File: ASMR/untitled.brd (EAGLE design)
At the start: 91 x 91 mm, 60 parts, among them J1 U.FL-R-SMT(01), J3 2172034-1, J4 POWER_JACKSLT, Q1 MMBT3904, Q2 MMBT3904, Q3 12MHz, Q4 MC-306, U2 DS1307Z+, U3 MAX3444EASA, U4 AMS1117, U5 MAX232CSE, X1 MSTBA2

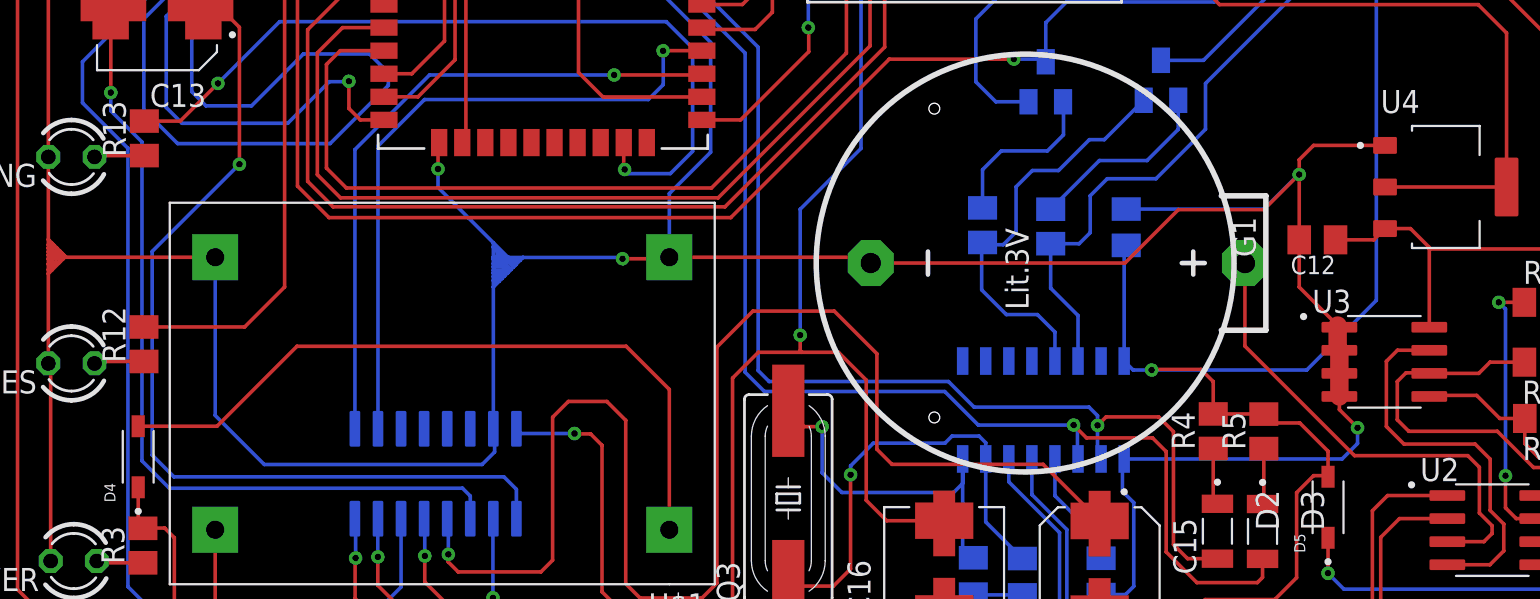
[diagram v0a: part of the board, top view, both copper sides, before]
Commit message: revisi .brd
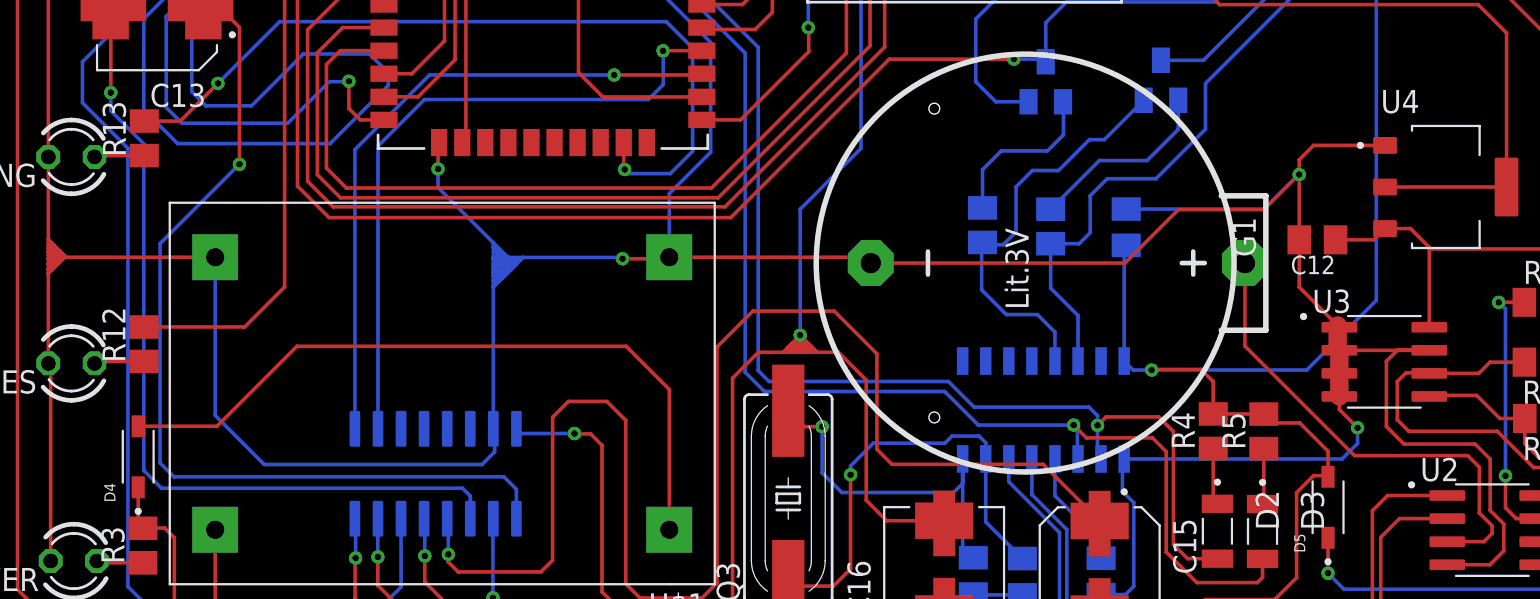
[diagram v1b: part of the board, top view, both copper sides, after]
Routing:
- net 3V3: track 234.7 -> 243.0 mm
- net GND: track 632.6 -> 636.9 mm
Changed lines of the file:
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@@
 <wire x1="66.064953125" y1="16.364715625" x2="66.064953125" y2="19.9532875" width="0.2" layer="1"/>
 <wire x1="66.064953125" y1="19.9532875" x2="66.675725" y2="20.564059375" width="0.2" layer="1"/>
-<wire x1="66.675725" y1="20.564059375" x2="68.422096875" y2="20.564059375" width="0.2" layer="1"/>
+<wire x1="66.675725" y1="20.564059375" x2="67.742509375" y2="20.564059375" width="0.2" layer="1"/>
+<wire x1="67.742509375" y1="20.564059375" x2="68.422096875" y2="20.564059375" width="0.2" layer="1"/>
 <wire x1="68.422096875" y1="20.564059375" x2="68.427296875" y2="20.558859375" width="0.2" layer="1"/>
 <wire x1="46.02720625" y1="7.0947875" x2="46.02720625" y2="6.58320625" width="0.2" layer="16"/>
@@
 <wire x1="19.6946625" y1="46.11838125" x2="19.945209375" y2="46.11838125" width="0.2" layer="16"/>
 <wire x1="19.945209375" y1="46.11838125" x2="20.063746875" y2="46.23691875" width="0.2" layer="16"/>
-<wire x1="63.477296875" y1="20.558859375" x2="68.427296875" y2="20.558859375" width="0" layer="19" extent="1-1"/>
+<wire x1="63.477296875" y1="20.558859375" x2="67.737309375" y2="20.558859375" width="0.2" layer="1"/>
+<wire x1="67.737309375" y1="20.558859375" x2="67.742509375" y2="20.564059375" width="0.2" layer="1"/>
 </signal>
 <signal name="USB_P">
@@
 <wire x1="38.556709375" y1="11.177509375" x2="37.4314125" y2="12.30280625" width="0.2" layer="1"/>
 <wire x1="37.4314125" y1="18.922815625" x2="35.904071875" y2="20.45015625" width="0.2" layer="1"/>
-<wire x1="35.904071875" y1="20.45015625" x2="33.8959" y2="20.45015625" width="0.2" layer="1"/>
-<wire x1="33.8959" y1="20.45015625" x2="31.49139375" y2="20.45015625" width="0.2" layer="1"/>
+<wire x1="35.904071875" y1="20.45015625" x2="34.738465625" y2="20.45015625" width="0.2" layer="1"/>
+<wire x1="34.738465625" y1="20.45015625" x2="33.8959" y2="20.45015625" width="0.2" layer="1"/>
+<wire x1="33.8959" y1="20.45015625" x2="33.685965625" y2="20.45015625" width="0.2" layer="1"/>
+<wire x1="33.685965625" y1="20.45015625" x2="33.501034375" y2="20.45015625" width="0.2" layer="1"/>
+<wire x1="33.501034375" y1="20.45015625" x2="33.320215625" y2="20.45015625" width="0.2" layer="1"/>
+<wire x1="33.320215625" y1="20.45015625" x2="33.1846" y2="20.45015625" width="0.2" layer="1"/>
+<wire x1="33.1846" y1="20.45015625" x2="32.853134375" y2="20.45015625" width="0.2" layer="1"/>
+<wire x1="32.853134375" y1="20.45015625" x2="31.49139375" y2="20.45015625" width="0.2" layer="1"/>
 <wire x1="31.49139375" y1="20.45015625" x2="30.0717" y2="19.0304625" width="0.2" layer="1"/>
 <wire x1="30.0717" y1="19.0304625" x2="30.0717" y2="6.275275" width="0.2" layer="1"/>
@@
 <wire x1="18.4332" y1="15.97845625" x2="18.173340625" y2="16.238315625" width="0.2" layer="16"/>
 <wire x1="33.8959" y1="20.45015625" x2="33.7958" y2="20.55025625" width="0.2" layer="1"/>
-<wire x1="33.7958" y1="20.55025625" x2="33.7958" y2="21.392821875" width="0.2" layer="1"/>
+<wire x1="33.7958" y1="20.55025625" x2="33.7958" y2="20.76345625" width="0.2" layer="1"/>
 <via x="33.7958" y="21.392821875" extent="1-16" drill="0.35"/>
+<wire x1="33.7958" y1="20.76345625" x2="33.7958" y2="21.392821875" width="0.2" layer="1"/>
 <wire x1="33.7958" y1="21.392821875" x2="33.7958" y2="28.324503125" width="0.2" layer="16"/>
 <wire x1="33.7958" y1="28.324503125" x2="37.144934375" y2="31.6736375" width="0.2" layer="16"/>
@@
 <wire x1="58.911721875" y1="55.437096875" x2="58.857303125" y2="55.382678125" width="0.2" layer="1"/>
 <wire x1="58.857303125" y1="55.382678125" x2="58.857303125" y2="54.914934375" width="0.2" layer="1"/>
+<wire x1="33.7958" y1="21.392821875" x2="33.35955625" y2="20.956578125" width="0.2" layer="1"/>
+<wire x1="33.35955625" y1="20.956578125" x2="33.2712" y2="20.868221875" width="0.2" layer="1"/>
+<wire x1="33.2712" y1="20.868221875" x2="33.137640625" y2="20.7346625" width="0.2" layer="1"/>
+<wire x1="33.137640625" y1="20.7346625" x2="33.07805" y2="20.675071875" width="0.2" layer="1"/>
+<wire x1="33.07805" y1="20.675071875" x2="32.853134375" y2="20.45015625" width="0.2" layer="1"/>
+<wire x1="33.07805" y1="20.675071875" x2="33.07805" y2="20.55670625" width="0.2" layer="1"/>
+<wire x1="33.07805" y1="20.55670625" x2="33.1846" y2="20.45015625" width="0.2" layer="1"/>
+<wire x1="33.137640625" y1="20.7346625" x2="33.320215625" y2="20.5520875" width="0.2" layer="1"/>
+<wire x1="33.320215625" y1="20.5520875" x2="33.320215625" y2="20.45015625" width="0.2" layer="1"/>
+<wire x1="33.2712" y1="20.868221875" x2="33.501034375" y2="20.6383875" width="0.2" layer="1"/>
+<wire x1="33.501034375" y1="20.6383875" x2="33.501034375" y2="20.45015625" width="0.2" layer="1"/>
+<wire x1="33.35955625" y1="20.956578125" x2="33.484596875" y2="20.8315375" width="0.2" layer="1"/>
+<wire x1="33.484596875" y1="20.8315375" x2="33.56884375" y2="20.747290625" width="0.2" layer="1"/>
+<wire x1="33.56884375" y1="20.747290625" x2="33.685965625" y2="20.63016875" width="0.2" layer="1"/>
+<wire x1="33.685965625" y1="20.63016875" x2="33.685965625" y2="20.592225" width="0.2" layer="1"/>
+<wire x1="33.685965625" y1="20.592225" x2="33.685965625" y2="20.45015625" width="0.2" layer="1"/>
+<wire x1="33.7958" y1="21.392821875" x2="33.7958" y2="20.974246875" width="0.2" layer="1"/>
+<wire x1="33.56884375" y1="20.747290625" x2="33.7958" y2="20.974246875" width="0.2" layer="1"/>
+<wire x1="33.7958" y1="21.392821875" x2="33.7958" y2="21.142740625" width="0.2" layer="1"/>
+<wire x1="33.7958" y1="21.142740625" x2="33.484596875" y2="20.8315375" width="0.2" layer="1"/>
+<wire x1="33.7958" y1="21.392821875" x2="34.412409375" y2="20.7762125" width="0.2" layer="1"/>
+<wire x1="34.412409375" y1="20.7762125" x2="34.551103125" y2="20.63751875" width="0.2" layer="1"/>
+<wire x1="34.551103125" y1="20.63751875" x2="34.738465625" y2="20.45015625" width="0.2" layer="1"/>
+<wire x1="33.685965625" y1="20.592225" x2="34.505809375" y2="20.592225" width="0.2" layer="1"/>
+<wire x1="34.505809375" y1="20.592225" x2="34.551103125" y2="20.63751875" width="0.2" layer="1"/>
+<wire x1="33.7958" y1="20.76345625" x2="34.14623125" y2="20.76345625" width="0.2" layer="1"/>
+<wire x1="34.14623125" y1="20.76345625" x2="34.399653125" y2="20.76345625" width="0.2" layer="1"/>
+<wire x1="34.399653125" y1="20.76345625" x2="34.412409375" y2="20.7762125" width="0.2" layer="1"/>
+<wire x1="33.7958" y1="20.974246875" x2="33.935440625" y2="20.974246875" width="0.2" layer="1"/>
+<wire x1="33.935440625" y1="20.974246875" x2="34.14623125" y2="20.76345625" width="0.2" layer="1"/>
+<wire x1="33.7958" y1="21.392821875" x2="33.935440625" y2="21.25318125" width="0.2" layer="1"/>
+<wire x1="33.935440625" y1="21.25318125" x2="33.935440625" y2="20.974246875" width="0.2" layer="1"/>
 </signal>
 <signal name="N$12">
@@
 <wire x1="18.173340625" y1="12.908290625" x2="17.487634375" y2="13.593996875" width="0.2" layer="16"/>
 <wire x1="17.487634375" y1="13.593996875" x2="-0.6770875" y2="13.593996875" width="0.2" layer="16"/>
-<wire x1="-0.6770875" y1="13.593996875" x2="-1.87726875" y2="14.794178125" width="0.2" layer="16"/>
-<wire x1="-1.87726875" y1="14.794178125" x2="-1.87726875" y2="25.999846875" width="0.2" layer="16"/>
-<wire x1="-1.87726875" y1="25.999846875" x2="2.925103125" y2="30.80221875" width="0.2" layer="16"/>
+<wire x1="-0.6770875" y1="13.593996875" x2="-1.444428125" y2="14.3613375" width="0.2" layer="16"/>
+<wire x1="-1.444428125" y1="14.3613375" x2="-1.444428125" y2="26.4326875" width="0.2" layer="16"/>
+<wire x1="-1.444428125" y1="26.4326875" x2="2.925103125" y2="30.80221875" width="0.2" layer="16"/>
 <via x="2.925103125" y="30.80221875" extent="1-16" drill="0.35"/>
 <wire x1="2.925103125" y1="38.34308125" x2="1.9885875" y2="39.279596875" width="0.2" layer="1"/>
@@
 <wire x1="15.633340625" y1="11.288315625" x2="15.633340625" y2="12.54055625" width="0.2" layer="16"/>
 <wire x1="15.633340625" y1="12.54055625" x2="15.2060875" y2="12.967809375" width="0.2" layer="16"/>
-<wire x1="15.2060875" y1="12.967809375" x2="-0.93304375" y2="12.967809375" width="0.2" layer="16"/>
-<wire x1="-0.93304375" y1="12.967809375" x2="-2.439434375" y2="14.4742" width="0.2" layer="16"/>
-<wire x1="-2.439434375" y1="14.4742" x2="-2.439434375" y2="32.028171875" width="0.2" layer="16"/>
-<wire x1="-2.439434375" y1="32.028171875" x2="-4.15501875" y2="33.74375625" width="0.2" layer="16"/>
+<wire x1="15.2060875" y1="12.967809375" x2="-1.36586875" y2="12.967809375" width="0.2" layer="16"/>
+<wire x1="-1.36586875" y1="12.967809375" x2="-2.3375875" y2="13.939528125" width="0.2" layer="16"/>
+<wire x1="-2.3375875" y1="13.939528125" x2="-2.3375875" y2="31.926325" width="0.2" layer="16"/>
+<wire x1="-2.3375875" y1="31.926325" x2="-4.15501875" y2="33.74375625" width="0.2" layer="16"/>
 <wire x1="-4.15501875" y1="33.74375625" x2="-4.15501875" y2="34.744996875" width="0.2" layer="16"/>
 <via x="-4.15501875" y="34.744996875" extent="1-16" drill="0.35"/>
@@
 <mfgpreviewcolor name="substratecolor" color="0xFF786E46"/>
 </mfgpreviewcolors>
+<errors>
+</errors>
 </board>
 </drawing>
